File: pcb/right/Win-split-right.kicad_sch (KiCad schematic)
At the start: 172 parts, among them J2 Conn_01x04_Socket, U1 RP2040_ProMicro, U2 74AHCT1G125

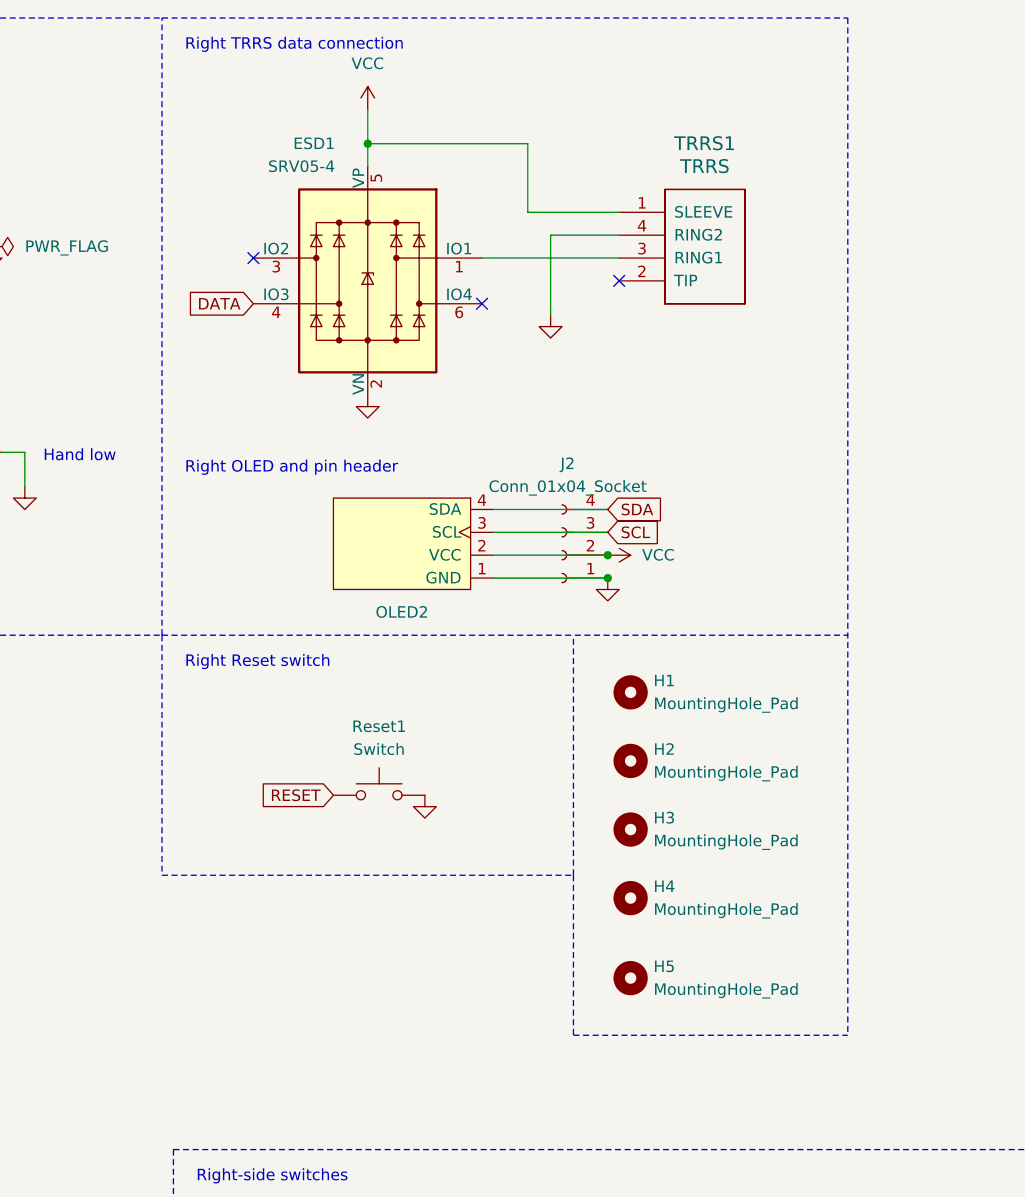
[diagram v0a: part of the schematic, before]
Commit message: prerouting right side
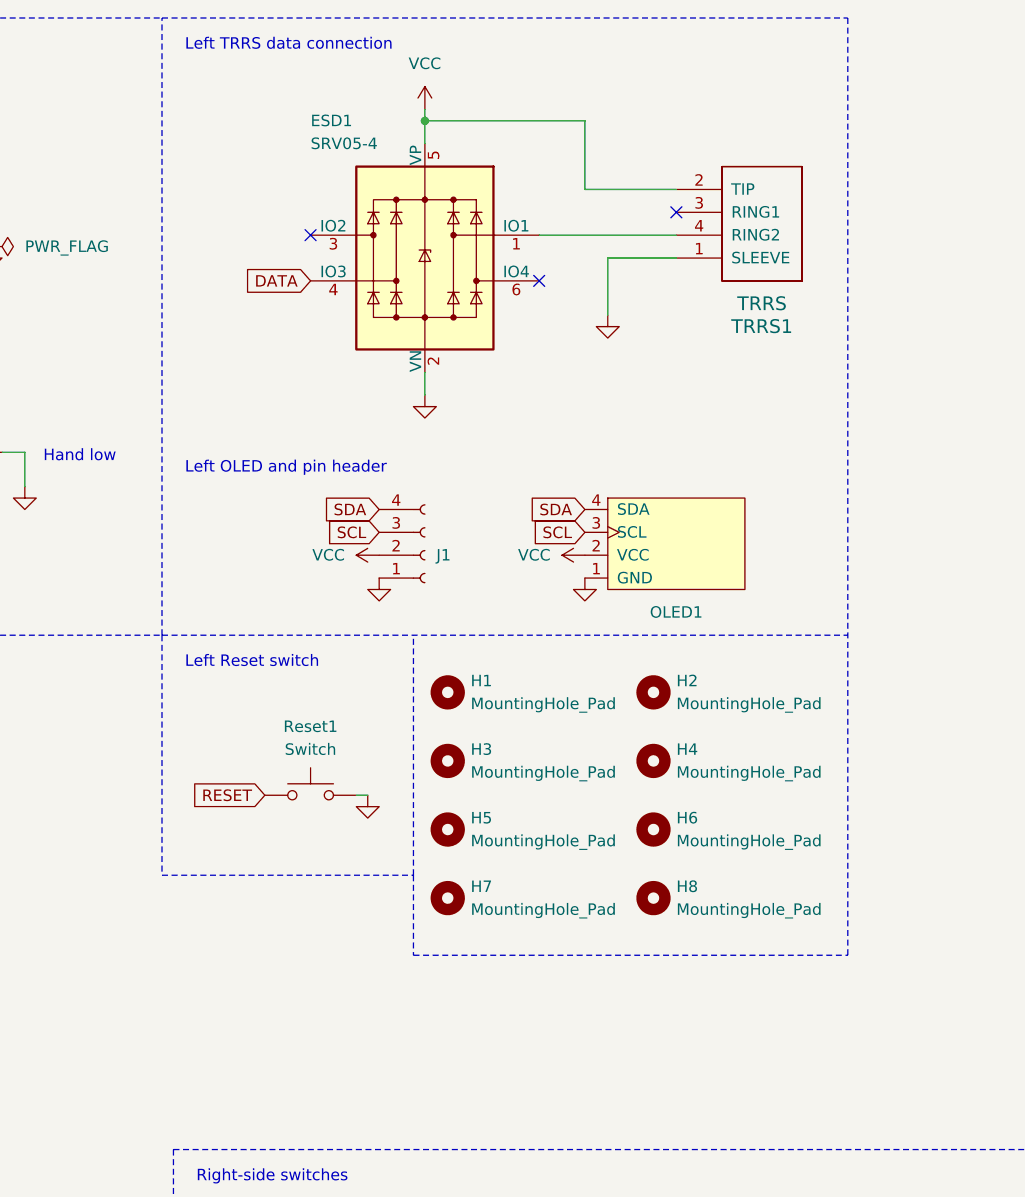
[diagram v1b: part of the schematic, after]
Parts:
- removed J2: Conn_01x04_Socket, Connector_PinHeader_2.54mm:PinHeader_1x04_P2.54mm_Vertical, symbol Connector:Conn_01x04_Socket
- removed OLED2: OLED_128x32, ScottoKeebs_Components:OLED_128x32, symbol ScottoKeebs:OLED_128x32
- added H6, H7, H8: MountingHole_Pad, winkeebs:HOLE_M2, symbol Mechanical:MountingHole
- added J1: Conn_01x04_Socket, Connector_PinHeader_2.54mm:PinHeader_1x04_P2.54mm_Vertical, symbol Connector:Conn_01x04_Socket
- added OLED1: OLED_128x32, ScottoKeebs_Components:OLED_128x32, symbol ScottoKeebs:OLED_128x32
- Reset1: LCSC (none) -> C231329
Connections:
- net GND: now also TRRS1.1 (SLEEVE), J1.1 (Pin_1), OLED1.1 (GND); no longer TRRS1.4 (RING2)
- net SCL: now also J1.3 (Pin_3), OLED1.3 (SCL)
- net SDA: now also J1.4 (Pin_4), OLED1.4 (SDA)
- net VCC: now also TRRS1.2 (TIP), J1.2 (Pin_2), OLED1.2 (VCC); no longer TRRS1.1 (SLEEVE)
- net at TRRS1.3 (RING1): no longer ESD1.1 (IO1)
- new net: ESD1.1 (IO1), TRRS1.4 (RING2)
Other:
- note added: "Left OLED and pin header"
- note added: "Left Reset switch"
- note added: "Left TRRS data connection"
- note removed: "Right OLED and pin header"
- note removed: "Right Reset switch"
- note removed: "Right TRRS data connection"
